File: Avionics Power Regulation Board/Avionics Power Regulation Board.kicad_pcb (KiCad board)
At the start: 2 copper layers, 127.4 x 80.5 mm, 57 parts, among them J1 Conn_01x05_Socket, Q1 NMOS, Q2 NMOS, Q3 NMOS, SW1 SW_Push, U1 LM2576HVS-5, U2 BQ76920PW, U4 TPS61085DGK

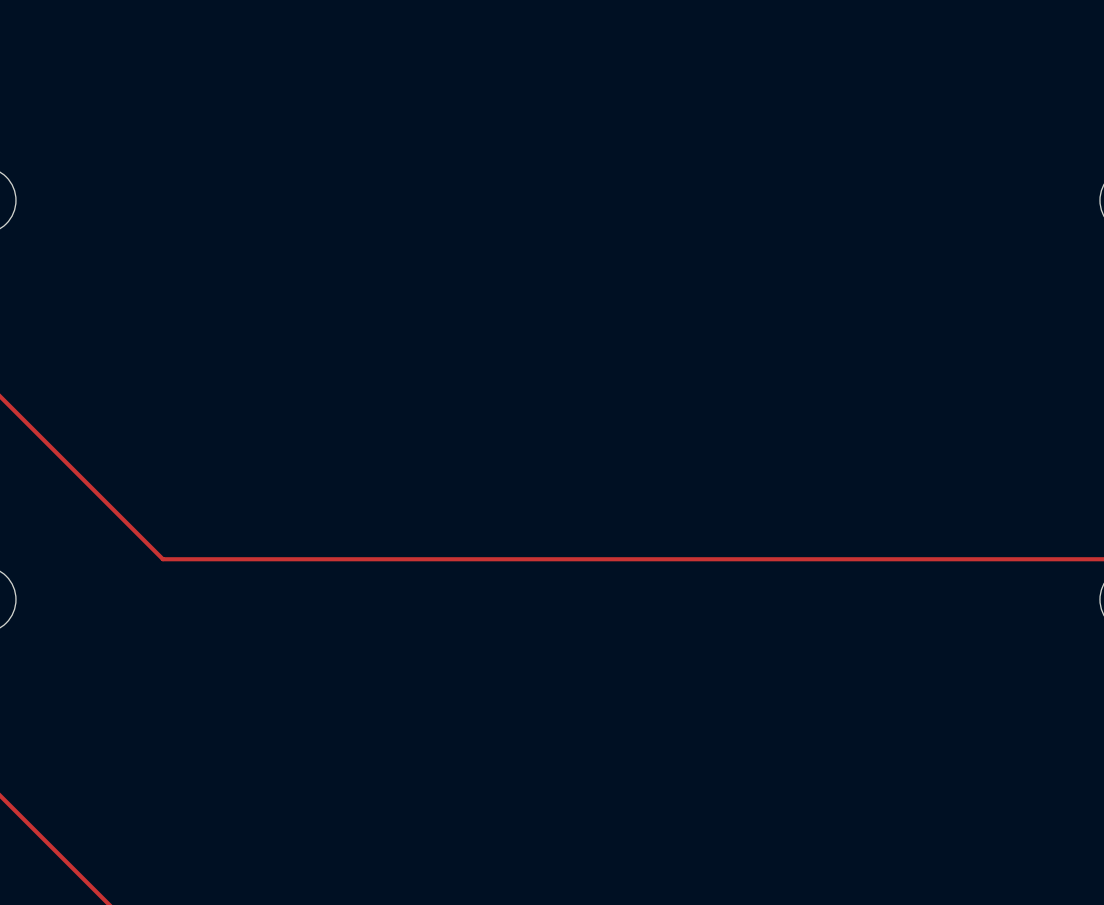
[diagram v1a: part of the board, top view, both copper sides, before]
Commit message: Miku
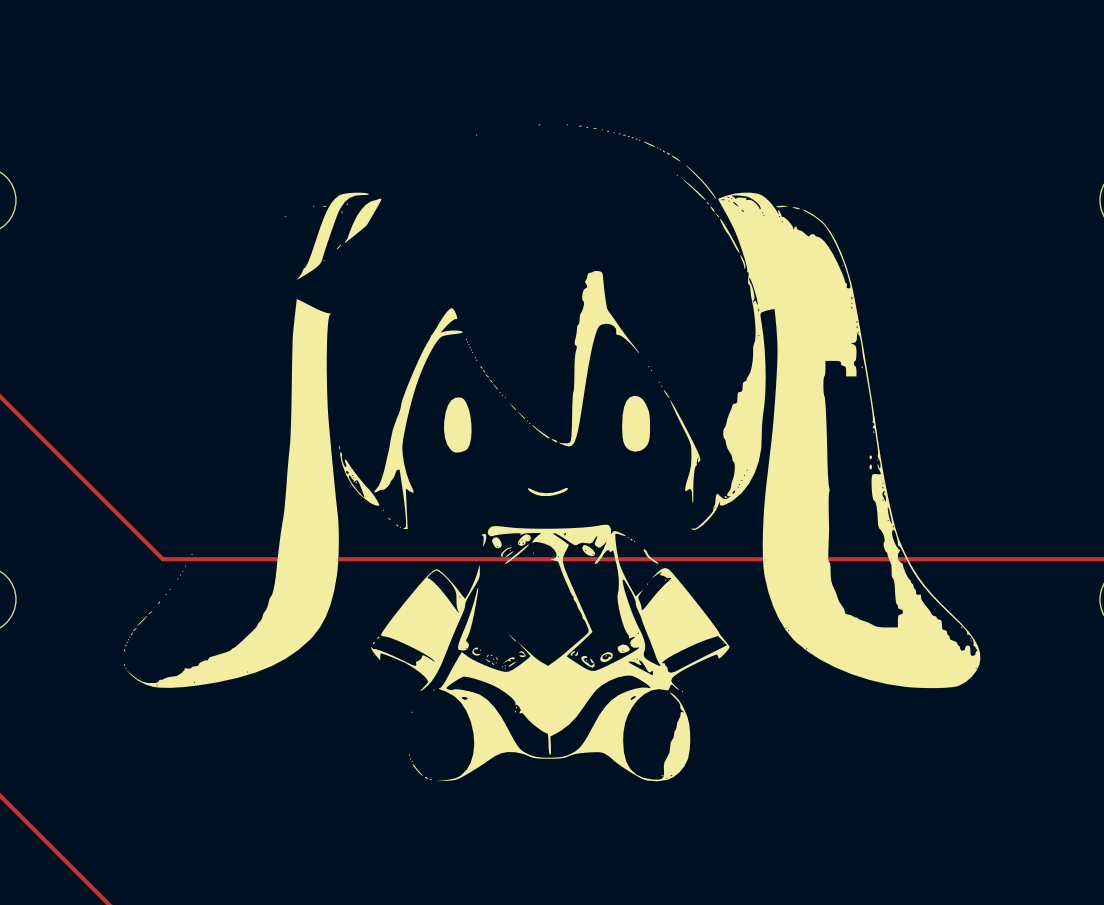
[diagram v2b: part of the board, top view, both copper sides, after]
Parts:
- added G***: LOGO, Miku:Miku, F.Cu at (123.8, 95.7)
